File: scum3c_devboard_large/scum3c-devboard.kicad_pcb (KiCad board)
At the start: 2 copper layers, 39.3 x 76.2 mm, 62 parts, among them J1 CONSMA001-SMD-G-T, J2 47346-0001, J3 Conn_02x06_Odd_Even, J4 Conn_01x23, J5 Conn_02x02_Odd_Even, J6 Conn_02x02_Odd_Even, U1 Perfboard, U2 FT231XS-U, U3 74AVC1T45GS,132, U4 74AVC1T45GS,132, U5 LP5907MFX-1.5, U6 S-85S1AB10-I6T1U, U7 S-85S1AB15-I6T1U, U8 scum3, U9AB1 MPU-9250

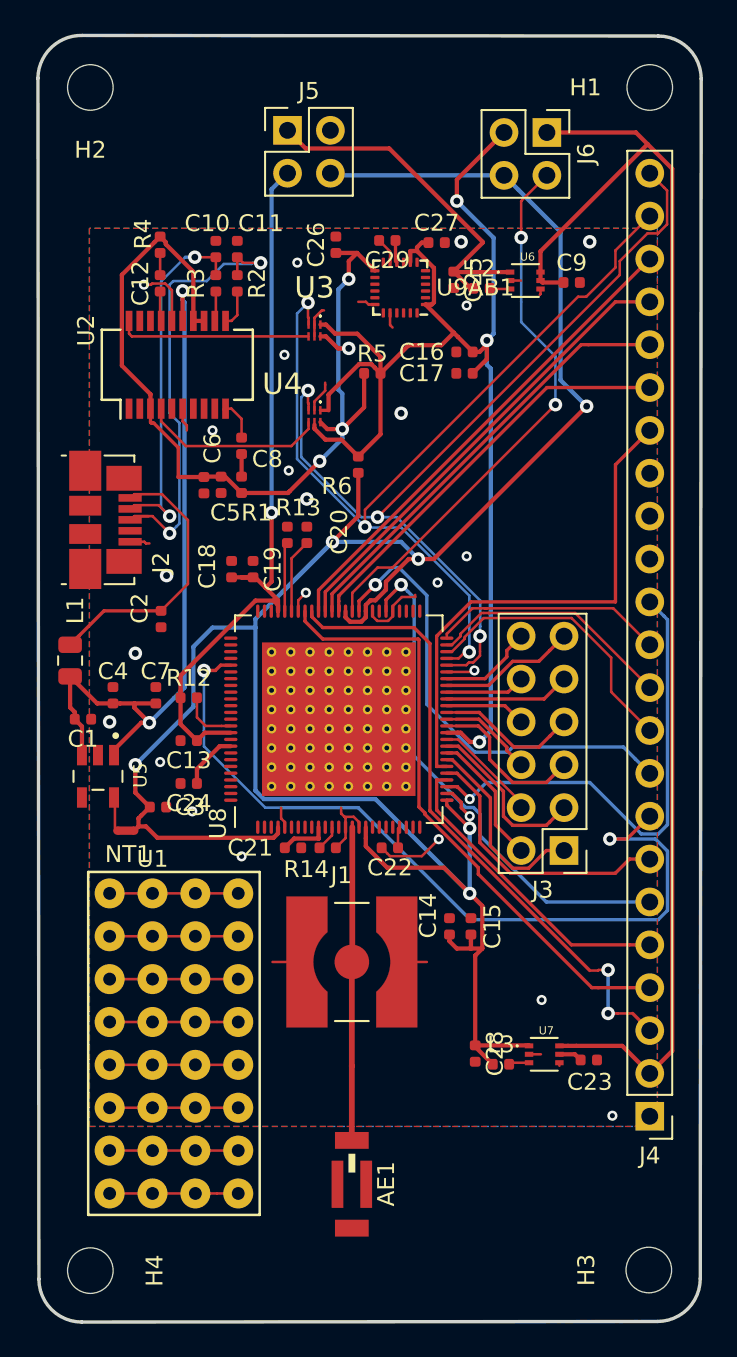
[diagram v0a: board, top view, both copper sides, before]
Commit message: ready for merge
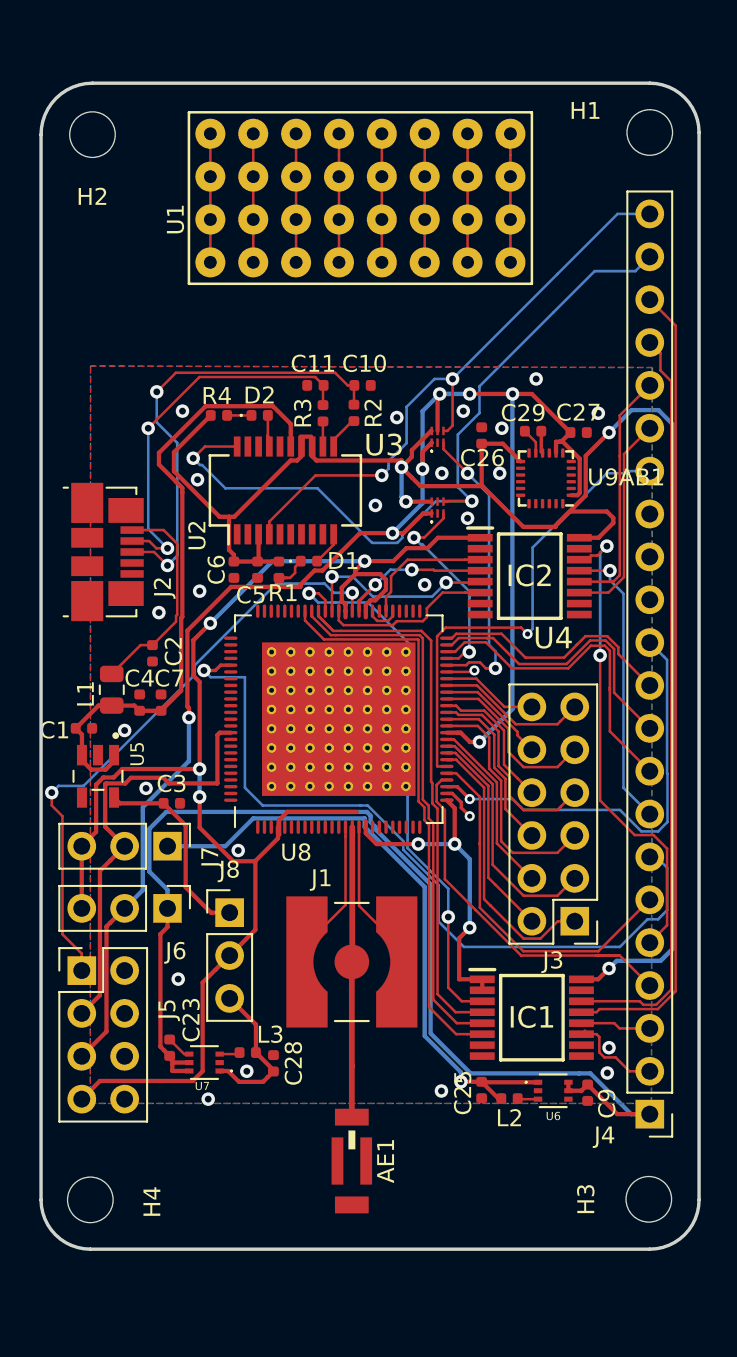
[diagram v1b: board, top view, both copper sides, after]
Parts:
- removed C12, C8: LED, Capacitor_SMD:C_0402_1005Metric
- removed C13, C14, C15, C16, C17, C18, C19, C20, C21, C22, C24: NP, Capacitor_SMD:C_0402_1005Metric
- removed NT1: Net-Tie_2, NetTie:NetTie-2_SMD_Pad0.5mm
- removed R12, R13, R14, R5, R6: NP, Resistor_SMD:R_0402_1005Metric
- added D1: LED, LED_SMD:LED_0402_1005Metric, F.Cu at (209.9, 95.6)
- added D2: LED, LED_SMD:LED_0402_1005Metric, F.Cu at (207.0, 87.0)
- added IC1: 74AVC4TD245PW,118, SamacSys_Parts:SOP65P640X110-16N, F.Cu at (223.1, 122.7)
- added IC2: 74AVC4TD245PW,118, SamacSys_Parts:SOP65P640X110-16N, F.Cu at (223.0, 96.5)
- added J7: Conn_01x03, Connector_PinHeader_2.54mm:PinHeader_1x03_P2.54mm_Vertical, F.Cu at (201.5, 112.5)
- added J8: Conn_01x03, Connector_PinHeader_2.54mm:PinHeader_1x03_P2.54mm_Vertical, F.Cu at (205.2, 116.5)
- H1, H2, H3, H4: footprint MountingHole:MountingHole_2.7mm -> MountingHole:MountingHole_2.7mm_M2.5
- J4: value Conn_01x23 -> Conn_01x22; footprint Connector_PinHeader_2.54mm:PinHeader_1x23_P2.54mm_Vertical -> Connector_PinHeader_2.54mm:PinHeader_1x22_P2.54mm_Vertical
- J5: value Conn_02x02_Odd_Even -> Conn_02x04_Odd_Even; footprint Connector_PinHeader_2.54mm:PinHeader_2x02_P2.54mm_Vertical -> Connector_PinHeader_2.54mm:PinHeader_2x04_P2.54mm_Vertical
- J6: value Conn_02x02_Odd_Even -> Conn_01x03; footprint Connector_PinHeader_2.54mm:PinHeader_2x02_P2.54mm_Vertical -> Connector_PinHeader_2.54mm:PinHeader_1x03_P2.54mm_Vertical
- moved J5 51.3 mm to (196.5, 119.9)
- moved J6 51.2 mm to (201.5, 116.2)
- moved C25 48.0 mm to (220.2, 127.0)
- moved L2 48.0 mm to (221.8, 127.5)
- moved U6 48.0 mm to (224.4, 127.0)
- moved C9 48.0 mm to (226.4, 127.1), turned to 270 degrees
- moved U1 37.4 mm to (201.5, 75.4), turned to 90 degrees
- moved C23 24.8 mm to (201.7, 124.5), turned to 90 degrees
- moved U7 20.1 mm to (203.7, 125.3), turned to 180 degrees
- moved L3 15.0 mm to (206.3, 124.7), turned to 180 degrees
- moved C26 14.2 mm to (220.2, 88.2)
- moved C29 14.2 mm to (223.2, 87.9)
- moved U9AB1 14.2 mm to (224.0, 90.7)
- moved C27 14.1 mm to (225.9, 88.0)
- moved U3 12.8 mm to (217.6, 92.5), turned to 0 degrees
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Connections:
- C28 pad 1: +VBAT -> /VBAT_TEENSY
- C3 pad 1: +VBAT -> /VBAT_USB
- J4 pad 1: GND -> +VIN
- J4 pad 10: /3WB_CLK -> /3WB_ENB
- J4 pad 11: /3WB_ENB -> /3WB_DATA
- J4 pad 12: /3WB_DATA -> /GPIO0
- J4 pad 13: /GPIO0 -> GND
- J4 pad 14: GND -> Net-(J4-Pad14)
- J4 pad 16: Net-(J4-Pad16) -> /GPIO3
- J4 pad 17: /GPIO3 -> /Teensy Connections/aPHIb33
- J4 pad 18: /aPHIb -> /Teensy Connections/aPHI33
- J4 pad 19: /aPHI -> /Teensy Connections/aSCANOUT33
- J4 pad 2: +VIN -> /Teensy Connections/aSCSEL33
- J4 pad 20: /aSCANOUT -> /Teensy Connections/aLOAD33
- J4 pad 21: /aLOAD -> /Rx33
- J4 pad 22: /RsRx -> /Tx33
- J4 pad 3: /aSCANIN -> /Teensy Connections/aSCANIN33
- J4 pad 4: /aSCSEL -> /GPIO1
- J4 pad 5: /GPIO1 -> /Teensy Connections/Clock33
- J4 pad 6: /Clock -> /GPIO2
- J4 pad 7: /GPIO2 -> /sReset
- J4 pad 8: /sReset -> /Teensy Connections/hReset33
- J4 pad 9: /hReset -> /3WB_CLK
- J5 pad 1: /1Vin -> /Boot_Source_Sel
- J5 pad 4: +VBAT -> GND
- J6 pad 2: /Boot_Source_Sel -> +VDDIO
- J6 pad 3: +VDDIO -> +VBAT
- L3 pad 1: +VBAT -> /VBAT_TEENSY
- U2 pad 20: /UART/RsRx33 -> /Rx33
- U2 pad 4: /UART/RsTx33 -> /Tx33
- U3 pad 4: /UART/RsRx33 -> /Rx33
- U4 pad 4: /UART/RsTx33 -> /Tx33
- U5 pad 5: Net-(NT1-Pad1) -> /VBAT_USB
- U7 pad 1: +VBAT -> /VBAT_TEENSY
- U8 pad 10: +VDD25 -> Net-(U8-Pad10)
- U8 pad 12: /scumsheet/VDD_AO_DISABLE -> Net-(U8-Pad12)
- U8 pad 70: /scumsheet/AUX_LDO_OUTPUT -> Net-(U8-Pad70)
- U8 pad 71: /scumsheet/VDDD_DISABLE -> Net-(U8-Pad71)
- U8 pad 72: +VDDD -> Net-(U8-Pad72)
- U8 pad 92: +VDDAO -> Net-(U8-Pad92)
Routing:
- net +UART33: track 56.5 -> 107.1 mm
- net /Teensy Connections/aLOAD33: track 0.00 -> 47.7 mm
- net /Rx33: track 0.00 -> 45.2 mm, vias 0 -> 2
- net /Teensy Connections/aSCANOUT33: track 0.00 -> 44.3 mm
- net +VBAT: track 152.1 -> 108.5 mm, vias 6 -> 7
- net /RsRx: track 54.9 -> 12.2 mm, vias 3 -> 2
- net /Tx33: track 0.00 -> 36.0 mm, vias 0 -> 2
- net /RsTx: track 53.2 -> 17.7 mm, vias 3 -> 2
- net /Teensy Connections/Clock33: track 0.00 -> 28.5 mm, vias 0 -> 2
- net /Clock: track 30.7 -> 8.56 mm, vias 1 -> 0
- net /hReset: track 27.7 -> 8.57 mm, vias 1 -> 2
- net +VDDD: track 44.3 -> 25.8 mm, vias 1 -> 0
- net +VDDIO: track 79.4 -> 97.6 mm, vias 3 -> 7
- net /Teensy Connections/hReset33: track 0.00 -> 17.4 mm, vias 0 -> 1
- net +VIN: track 82.0 -> 66.4 mm
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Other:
- board size 39.3 x 76.2 mm -> 39 x 69.1 mm
